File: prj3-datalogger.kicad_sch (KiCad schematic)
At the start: 22 parts, among them U1 24LC1025, U2 24LC1025, U3 DS1337S_, U4 ATMEGA328P-AU, Y1 Crystal, Y2 Crystal

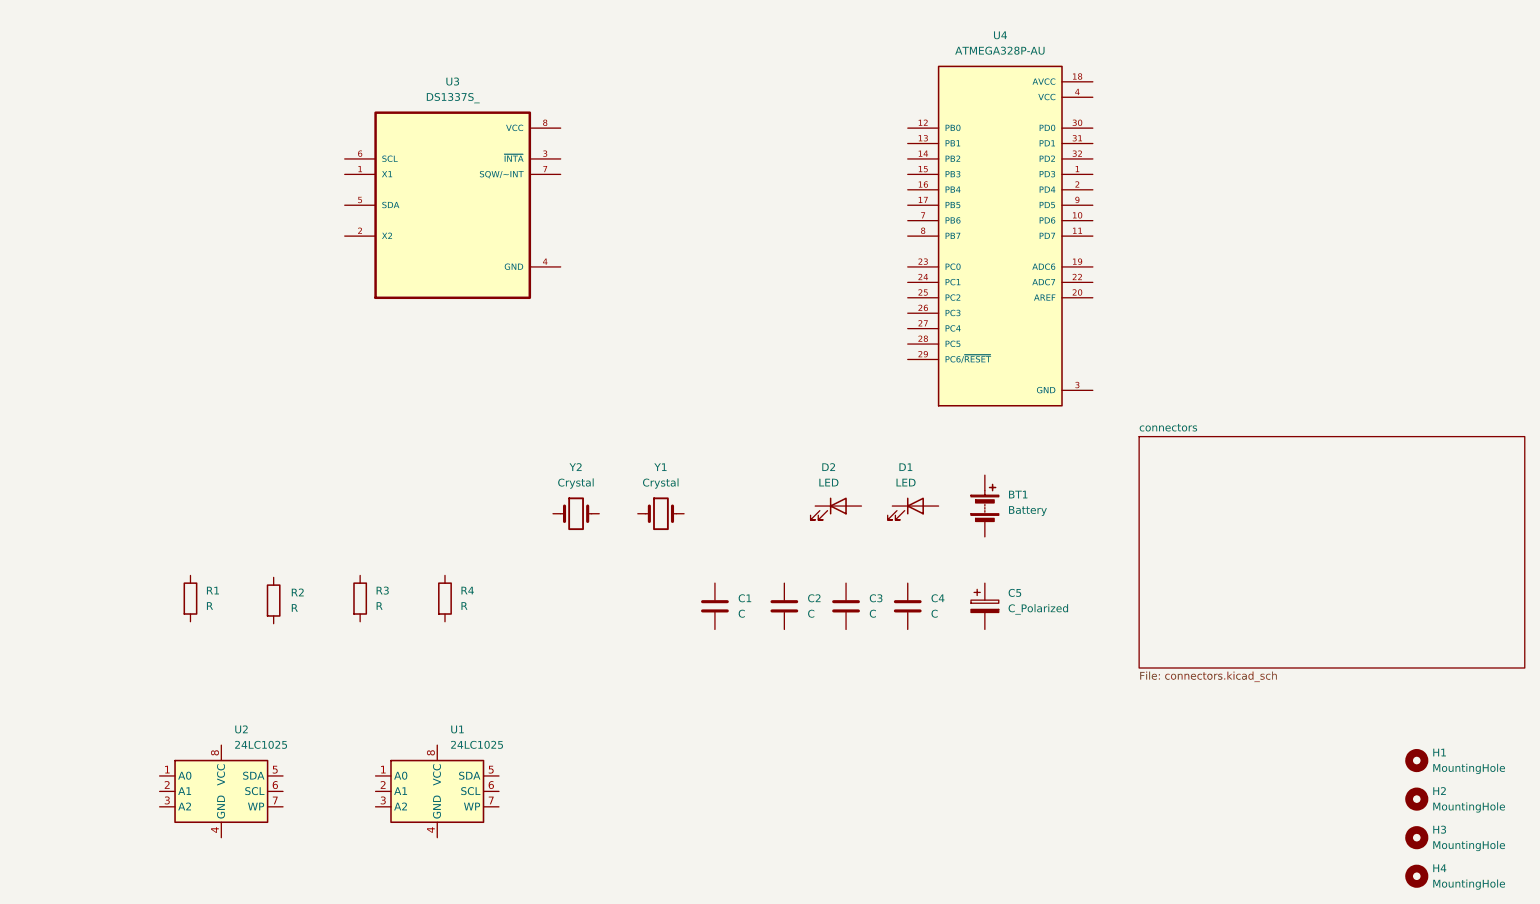
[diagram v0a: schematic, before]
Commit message: arranged symbols.
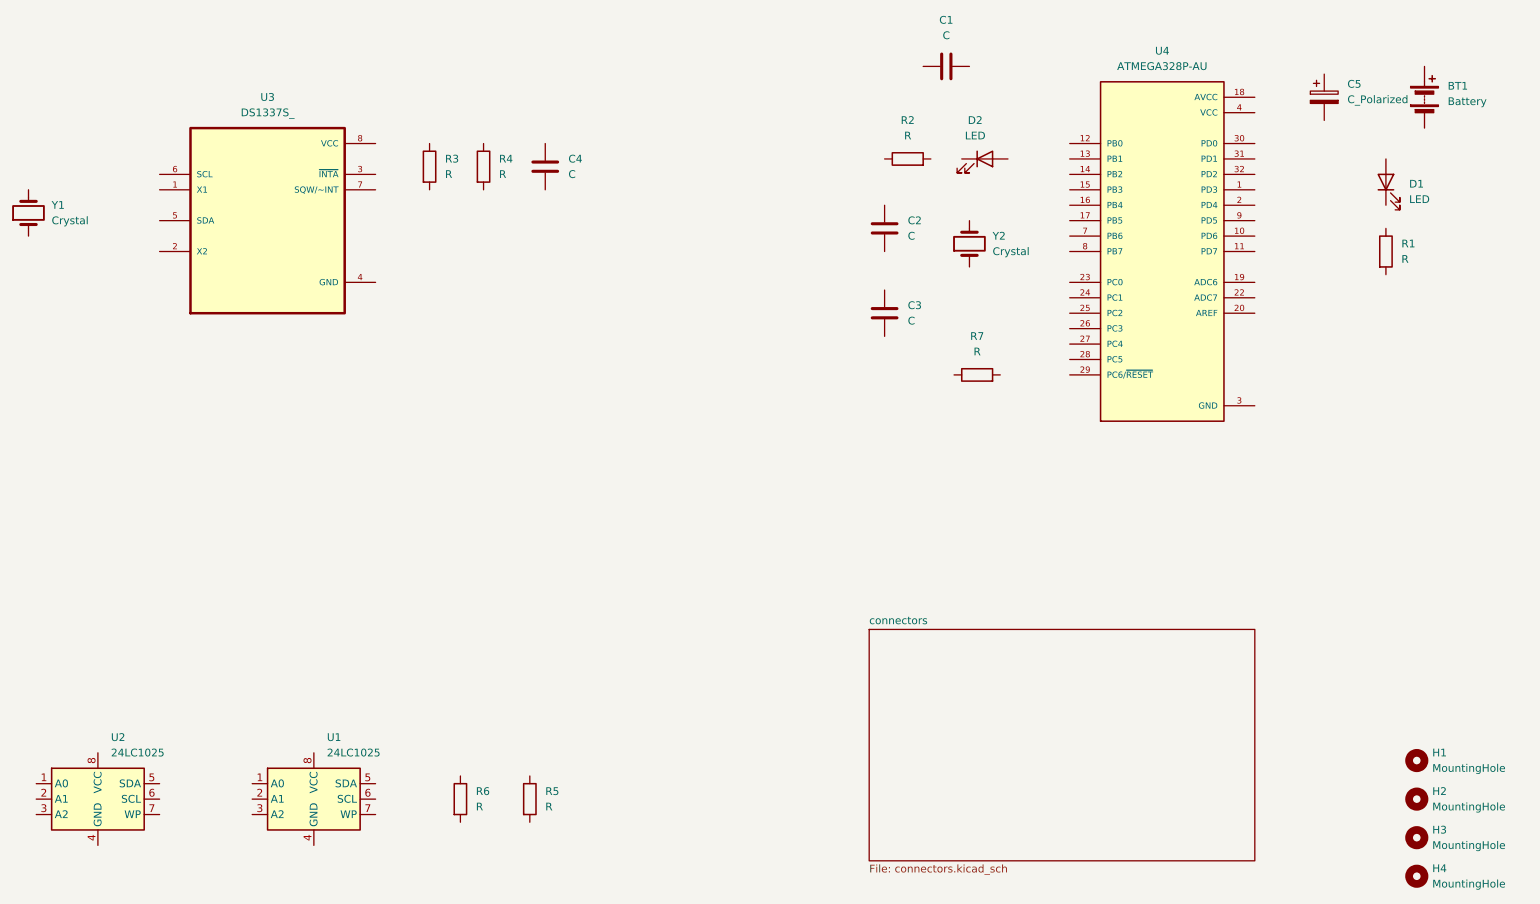
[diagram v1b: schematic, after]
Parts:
- added R5, R6, R7: R, symbol Device:R
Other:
- moved on the sheet: BT1, C1, C2, C3, C4, C5, D1, D2, R1, R2, R3, R4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
